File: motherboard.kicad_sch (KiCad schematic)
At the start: 19 parts, among them J1 NES Connector, U1 UM3304QT, U10 UM3304QT, U11 UM3304QT, U12 UM3304QT, U13 UM3304QT, U14 UM3304QT, U15 UM3304QT, U16 UM3304QT, U17 UM3304QT, U18 UM3304QT, U2 UM3304QT, U3 UM3304QT, U4 UM3304QT, U5 UM3304QT, U6 UM3304QT, U7 UM3304QT, U8 UM3304QT, U9 UM3304QT

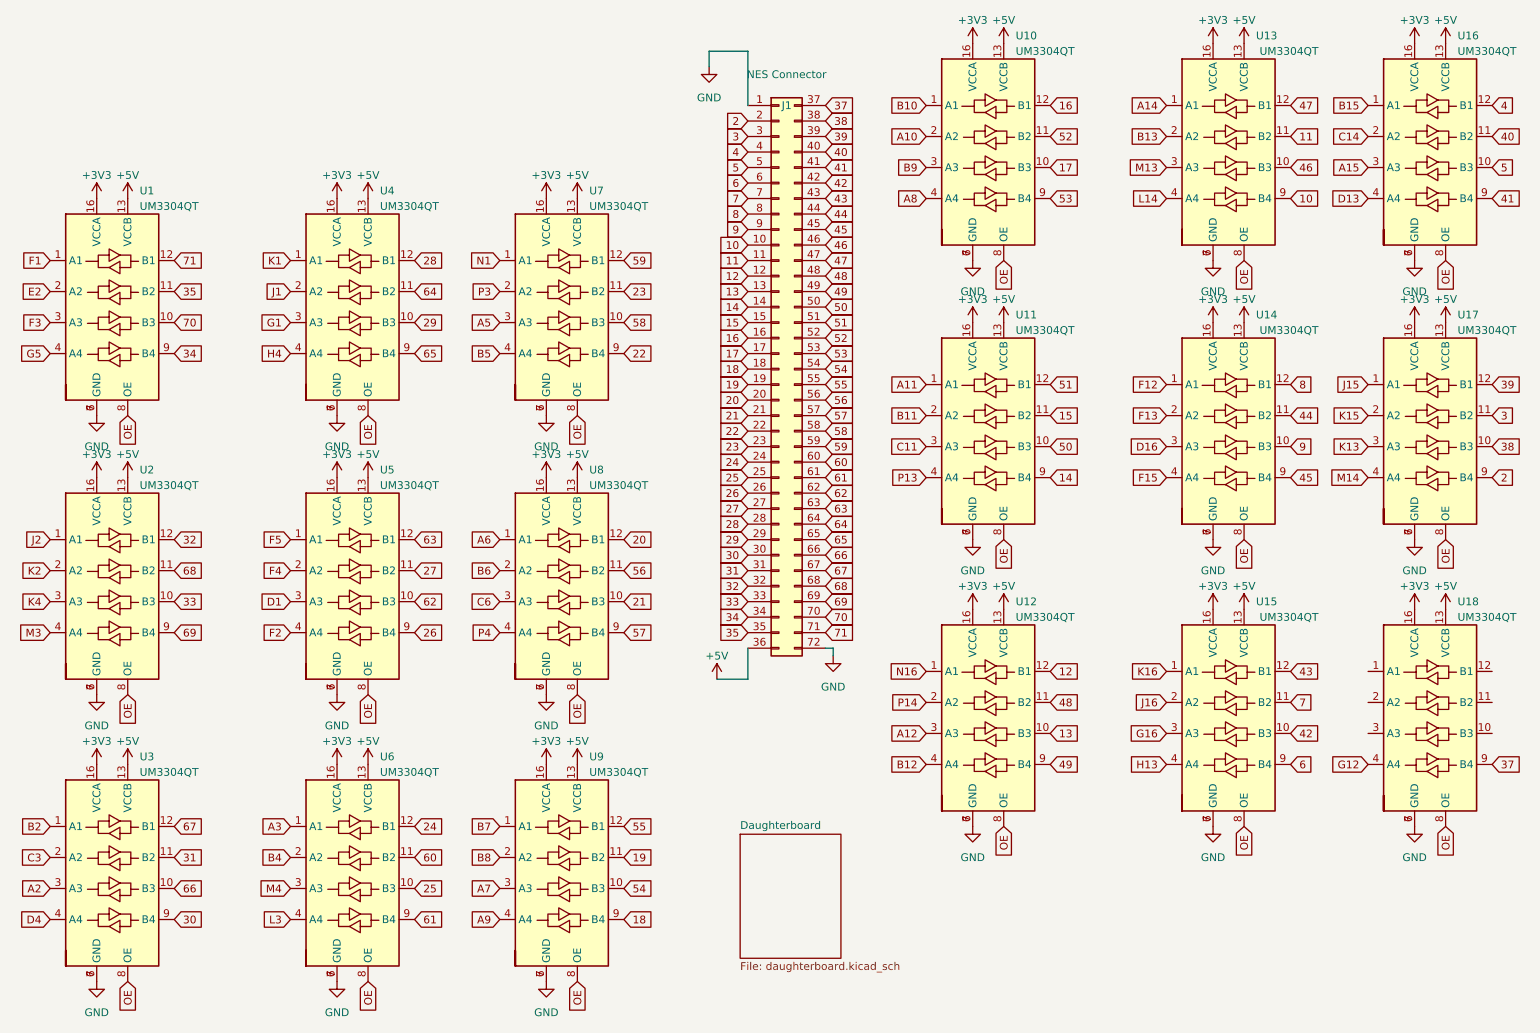
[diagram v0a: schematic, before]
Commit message: Possibly finished PCB
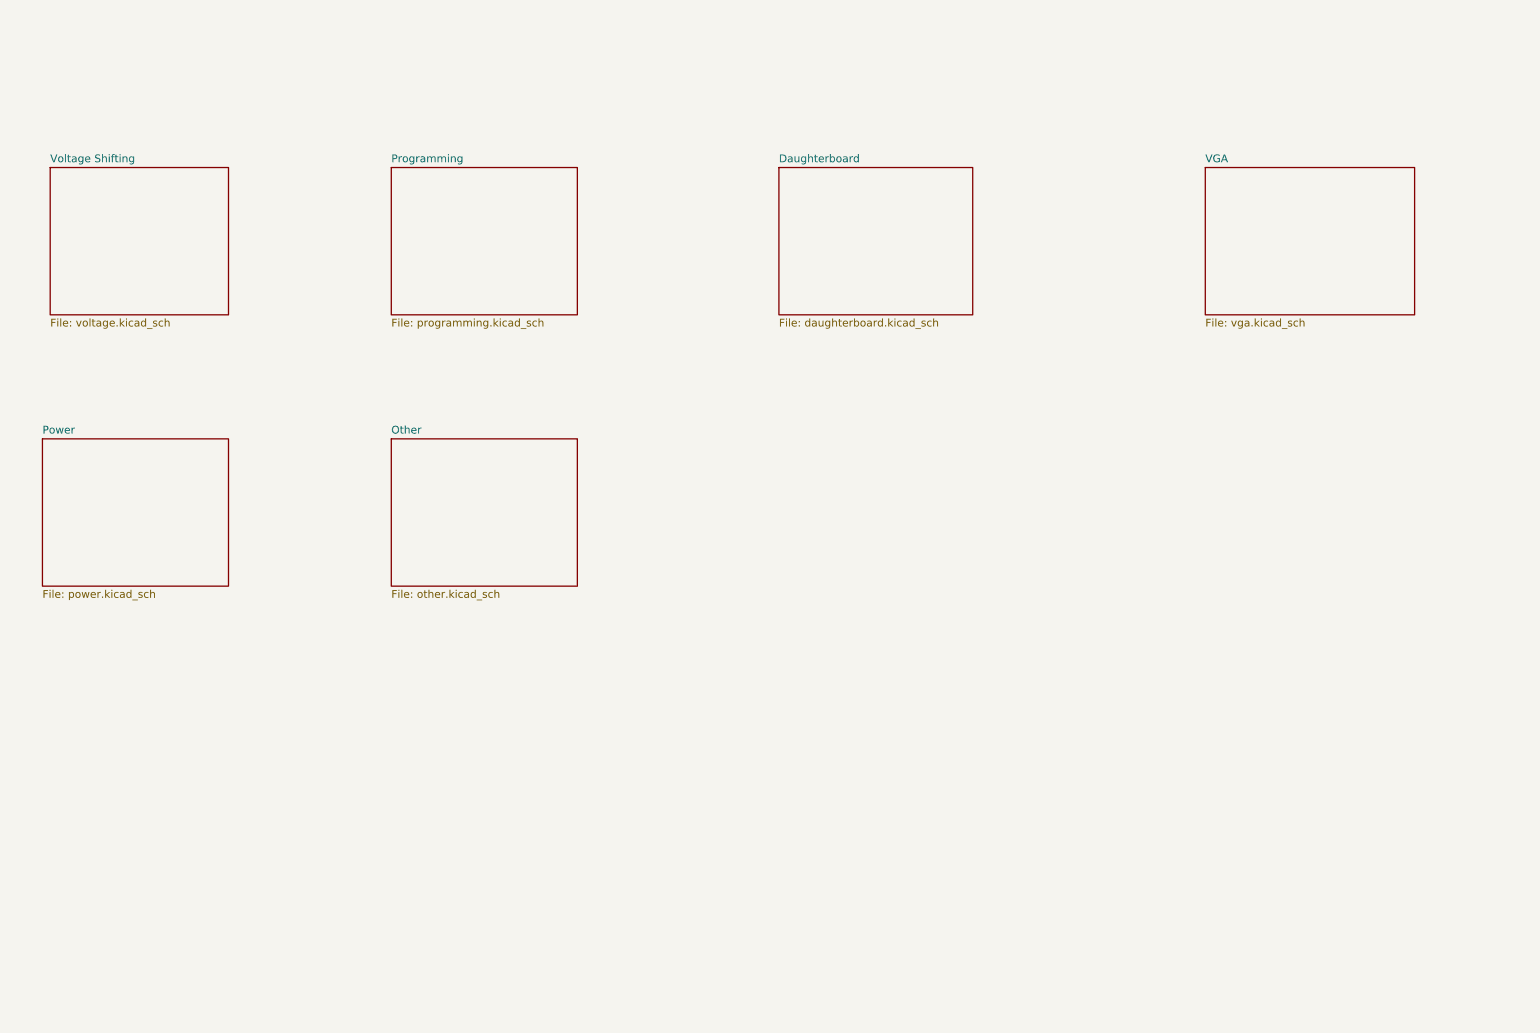
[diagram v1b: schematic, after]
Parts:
- removed J1: NES Connector, Library:NES_Connector, symbol Connector_Generic:Conn_02x36_Top_Bottom
- removed U1, U10, U11, U12, U13, U14, U15, U16, U17, U18, U2, U3, U4, U5, U6, U7, U8, U9: UM3304QT, Library:QFN-16_1.8x2.6_Pitch0.4mm, symbol New_Library:UM3304QT
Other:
- added sheet Other (other.kicad_sch)
- added sheet Power (power.kicad_sch)
- added sheet Programming (programming.kicad_sch)
- added sheet VGA (vga.kicad_sch)
- added sheet Voltage Shifting (voltage.kicad_sch)
